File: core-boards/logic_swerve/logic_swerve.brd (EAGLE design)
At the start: 143.2 x 130.9 mm, 75 parts, among them J1 5-PIN_2MM-H, J10 6-PIN_2MM-V, J11 6-PIN_2MM-V, J12 6-PIN_2MM-V, J13 5-PIN_2MM-H, J14 5-PIN_2MM-H, J15 B2PS-VH(LF)(SN), J16 S3B-VH, J17 B2PS-VH(LF)(SN), J2 5-PIN_2MM-H, J3 8-PIN_2MM-V, J4 6-PIN_2MM-V, J5 B2PS-VH(LF)(SN), J6 6-PIN_2MM-V, J7 B2PS-VH(LF)(SN), J8 B2PS-VH(LF)(SN), J9 B2PS-VH(LF)(SN), Q4 STT4P3LLH6, T1 R-78E5.0-1.0, U1 INA198AIDBVR, U2 INA198AIDBVR, U3 INA198AIDBVR, U4 TC4427ACOA713, U5 TXB0106PWRPW16-M, U6 MCP2551T-I/SN, U7 INA198AIDBVR, U8 TLV70233DBVR, U9 D5V0L1B2WS-7

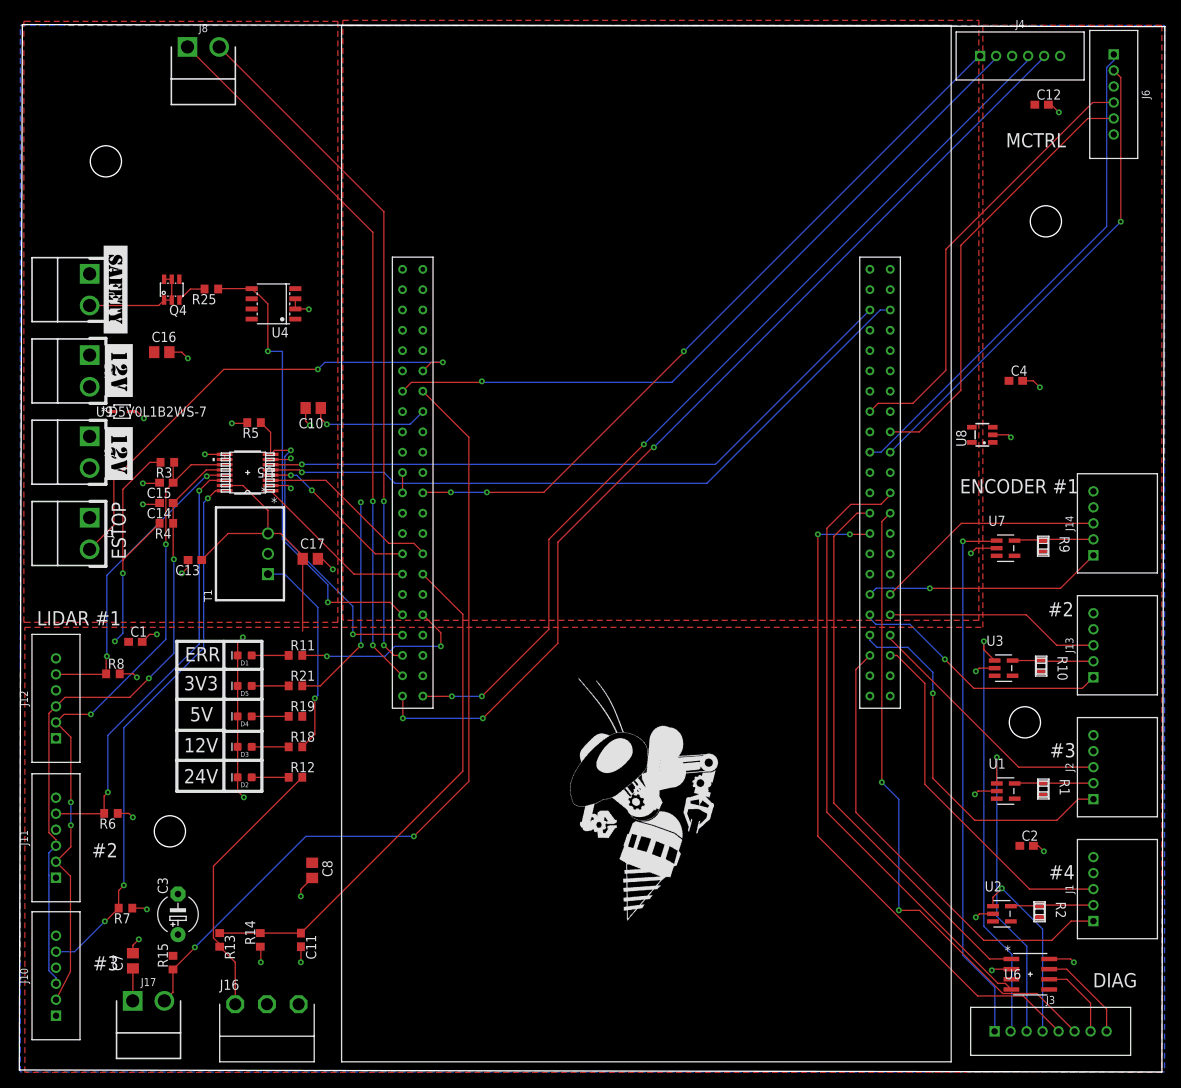
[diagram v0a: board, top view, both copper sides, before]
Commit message: Logic Swerve Board
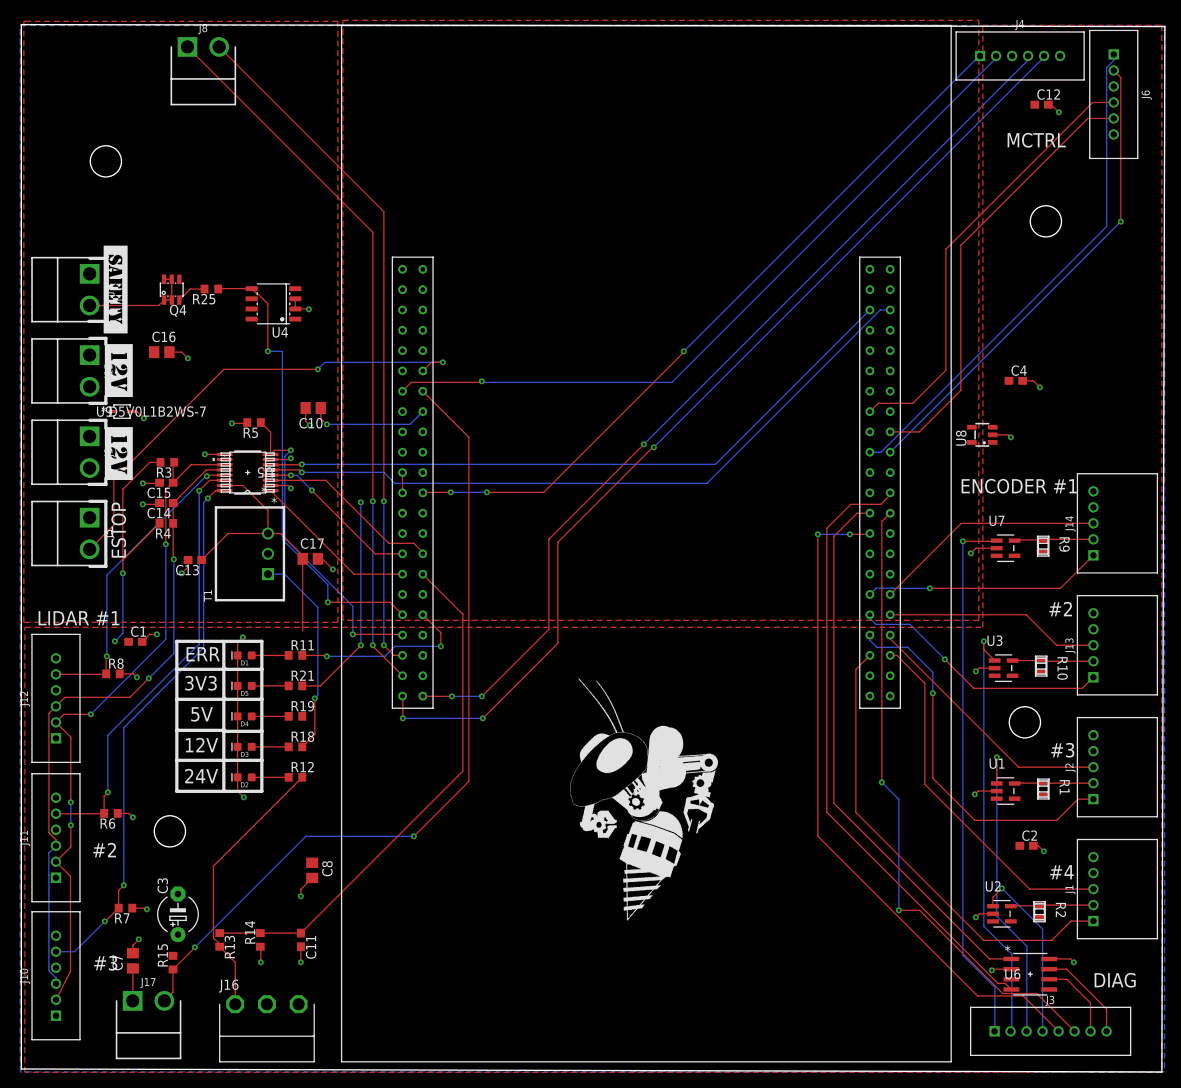
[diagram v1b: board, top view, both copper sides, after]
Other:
- board size 143.2 x 130.9 mm -> 142.9 x 130.9 mm
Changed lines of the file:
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@@
 <board>
 <plain>
-<wire x1="-113.94" y1="26.92" x2="28.88" y2="26.67" width="0" layer="20"/>
+<wire x1="-113.69" y1="27.045" x2="28.88" y2="26.67" width="0" layer="20"/>
 <wire x1="28.88" y1="26.67" x2="29.255" y2="157.345" width="0" layer="20"/>
-<wire x1="29.255" y1="157.345" x2="-113.565" y2="157.595" width="0" layer="20"/>
-<wire x1="-113.565" y1="157.595" x2="-113.94" y2="26.92" width="0" layer="20"/>
+<wire x1="29.255" y1="157.345" x2="-113.69" y2="157.595" width="0" layer="20"/>
+<wire x1="-113.69" y1="157.595" x2="-113.69" y2="27.045" width="0" layer="20"/>
 <wire x1="-88.25" y1="80.5" x2="-83.625" y2="80.5" width="0.4064" layer="21"/>
 <wire x1="-83.625" y1="80.5" x2="-83.625" y2="77" width="0.4064" layer="21"/>
